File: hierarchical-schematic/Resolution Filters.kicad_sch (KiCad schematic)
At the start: 50 parts, among them J501 In, J502 Terminal Block, J503 Out, K501 G5V-1, K502 G5V-1, SW501 SW_SPST, T501 Transformer_1P_1S, T502 Transformer_1P_1S, Y501 10.7MHz, Y502 10.7MHz, Y503 10.7MHz, Y504 10.7MHz

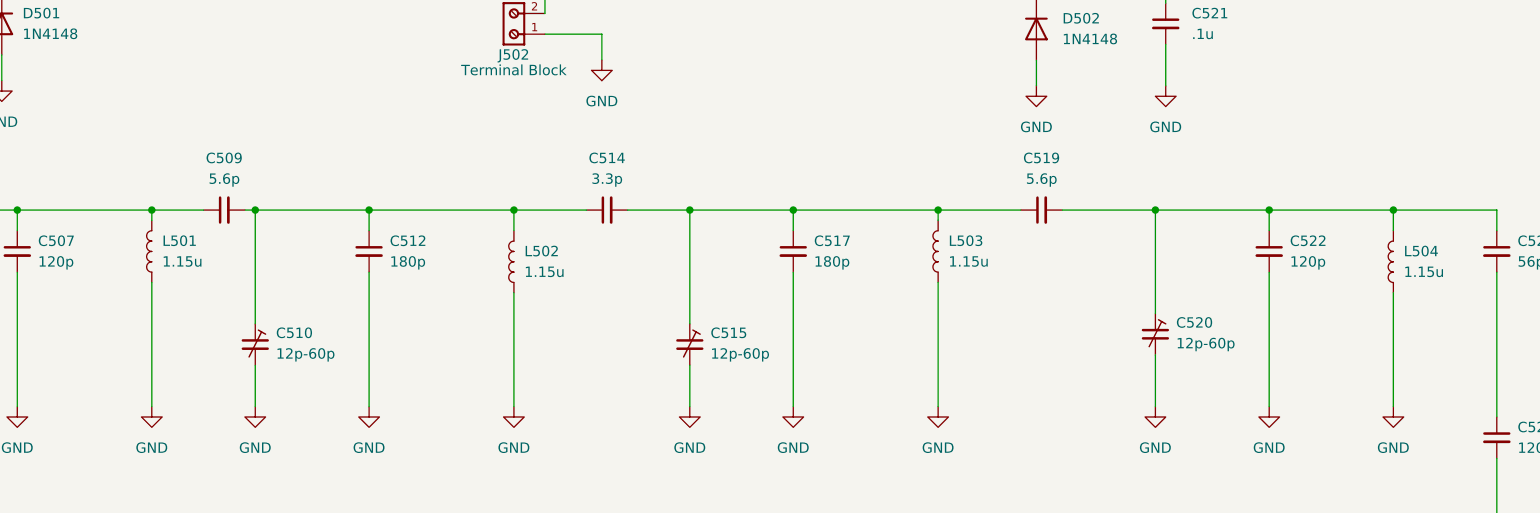
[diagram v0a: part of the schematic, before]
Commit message: v7 conversion
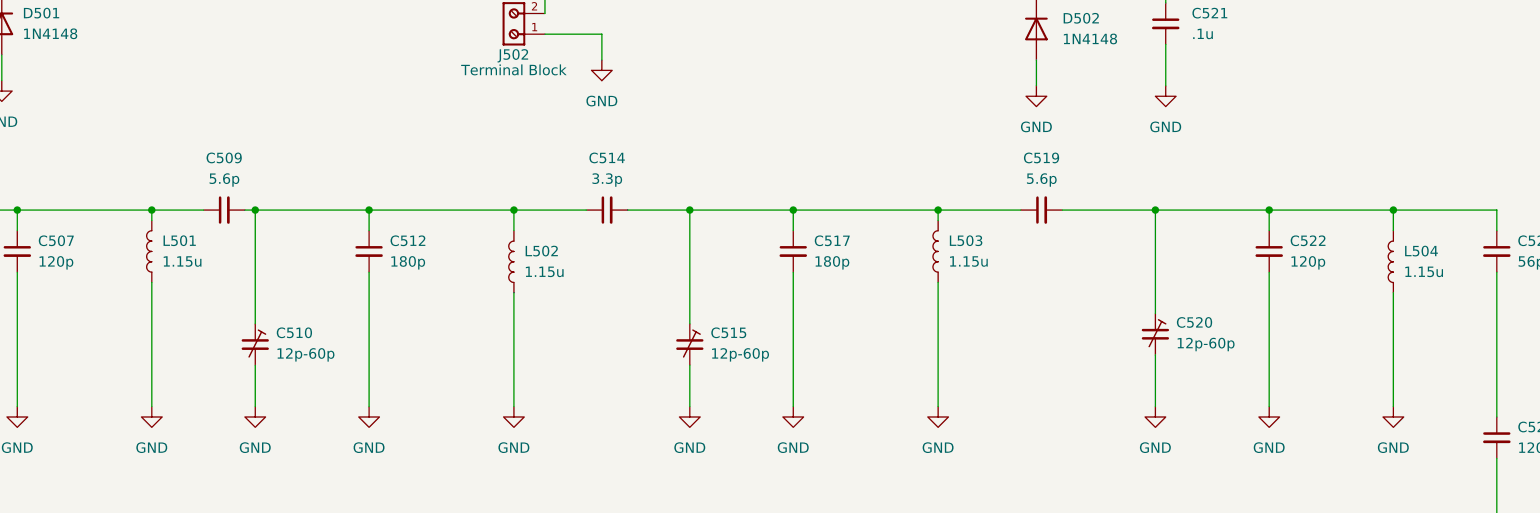
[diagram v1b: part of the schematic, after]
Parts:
- J501, J503: Spice_Model Conn_Coaxial -> (none); Spice_Netlist_Enabled N -> (none); Spice_Primitive J -> (none)
- J502: Spice_Model Terminal Block -> (none); Spice_Netlist_Enabled N -> (none); Spice_Primitive J -> (none)
